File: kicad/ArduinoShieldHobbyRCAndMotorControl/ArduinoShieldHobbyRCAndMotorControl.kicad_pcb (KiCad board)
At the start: 2 copper layers, 68.6 x 53.3 mm, 15 parts, among them J1 Power, J10 Conn_01x03_Socket, J11 Conn_01x03_Socket, J2 Digital/PWM, J3 Analog, J4 Digital/PWM, J5 Conn_01x03_Socket, J6 Conn_01x07_Pin, J7 Conn_01x03_Socket, J8 Conn_01x03_Socket, J9 Conn_01x03_Socket

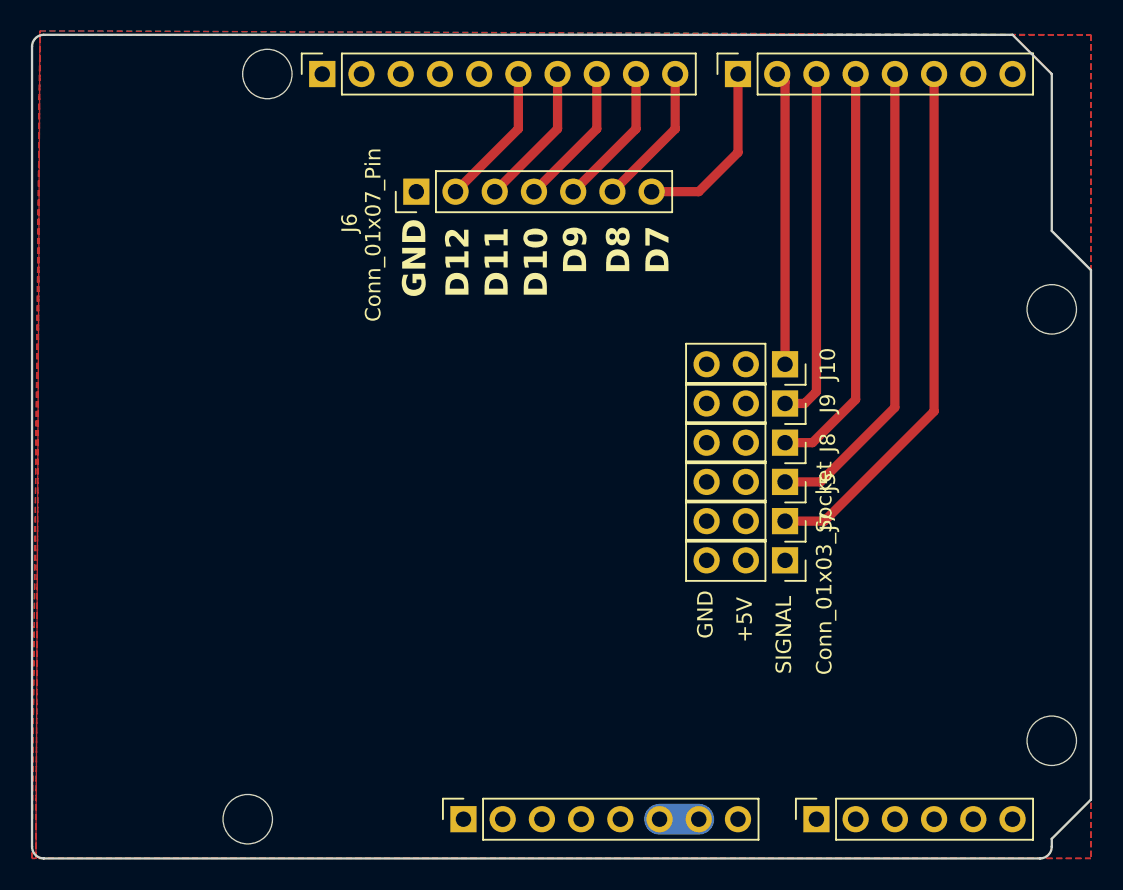
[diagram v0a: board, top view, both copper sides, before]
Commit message: added DesignCyberneticsNavigatingTheNew.pdf and Table_of_Mechanicks_Cyclopaedia_Volume_2.jpg
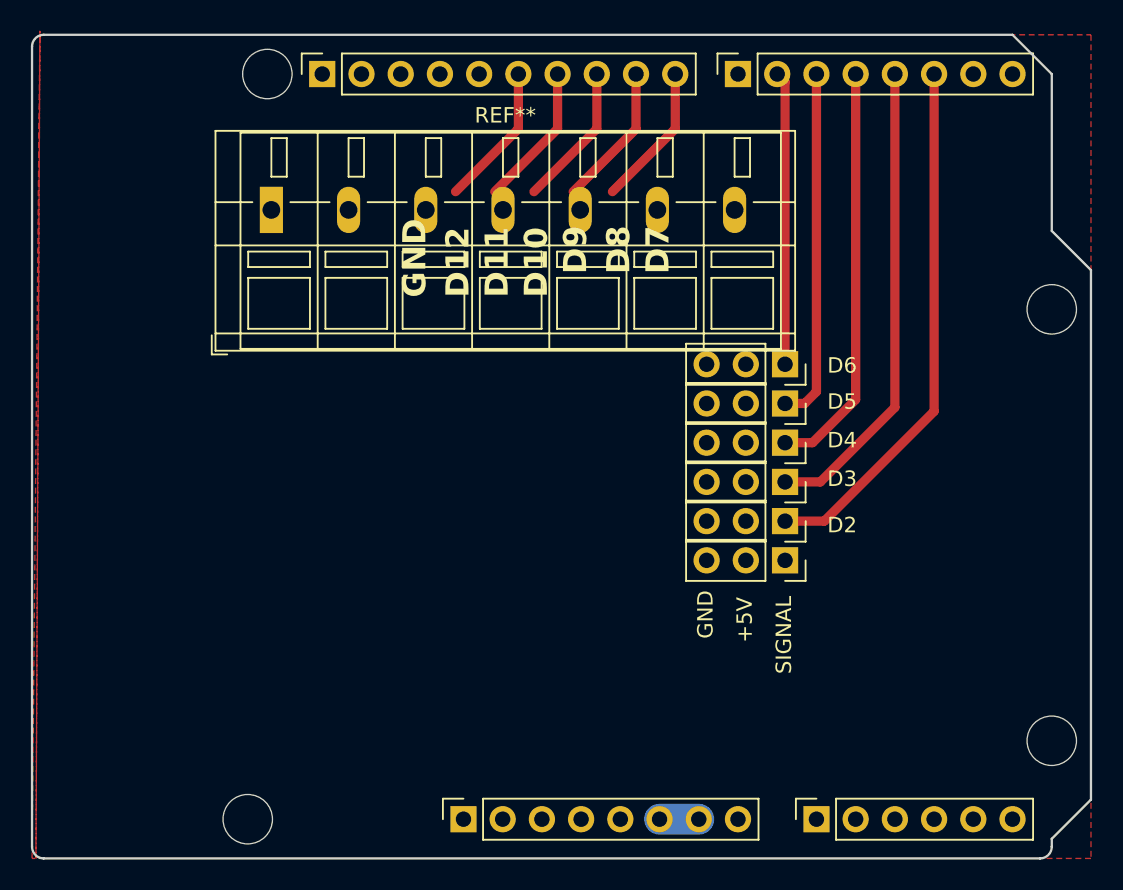
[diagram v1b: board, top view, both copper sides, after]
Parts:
- removed J6: Conn_01x07_Pin, Connector_PinHeader_2.54mm:PinHeader_1x07_P2.54mm_Vertical
- added REF**: TerminalBlock_WAGO_236-107_1x07_P5.00mm_45Degree, TerminalBlock_WAGO:TerminalBlock_WAGO_236-107_1x07_P5.00mm_45Degree, F.Cu at (115.5, 58.0)
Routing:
- net Net-(J4-Pin_1): track 11.7 -> 0.00 mm
- removed copper zone on B.Cu, net GND
- removed copper zone on F.Cu, net GND
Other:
- board text added: "D2"
- board text added: "D3"
- board text added: "D4"
- board text added: "D5"
- board text added: "D6"
